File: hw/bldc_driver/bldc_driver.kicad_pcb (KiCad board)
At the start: 4 copper layers, 101 x 48 mm, 150 parts, among them J1 430450412, J2 B4B-EH-A(LF)(SN), J3 B4B-EH-A(LF)(SN), J4 1733583, Q2 IRF540N, Q3 IRF540N, Q4 IRF540N, Q5 IRF540N, Q6 IRF540N, Q7 IRF540N, SW1 BTSA-N-P-1, U1 CH32V30xRxTx, U10 TPS54202DDC, U11 AMC1200BDWV, U12 AMC1200BDWV, U13 AMC1200BDWV, U14 SN65HVD230, U2 STGAP2SCM, U3 STGAP2SCM, U4 STGAP2SCM, U5 STGAP2SCM, U6 STGAP2SCM, U7 STGAP2SCM, U8 TPS54202DDC, U9 AMC1200BDWV, Y1 Crystal_GND24

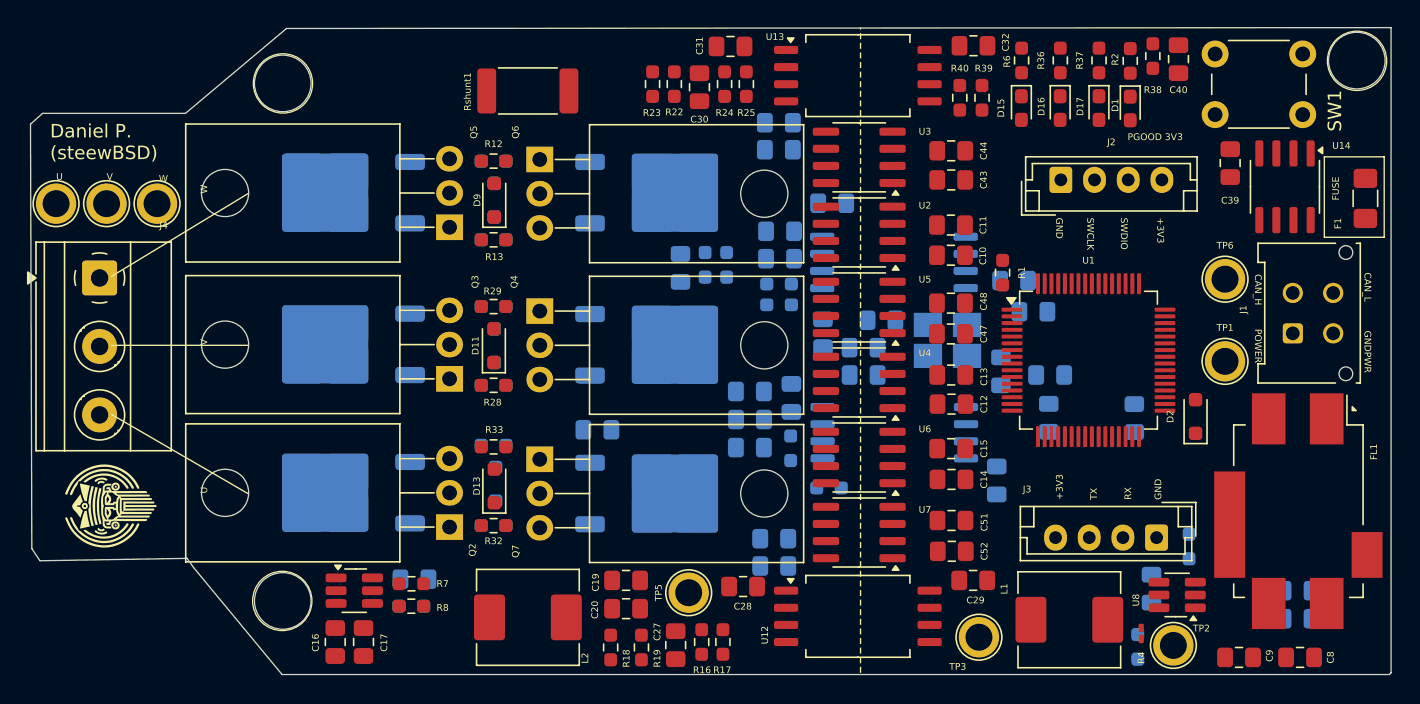
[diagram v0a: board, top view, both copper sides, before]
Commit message: bldc: pre-routing commit
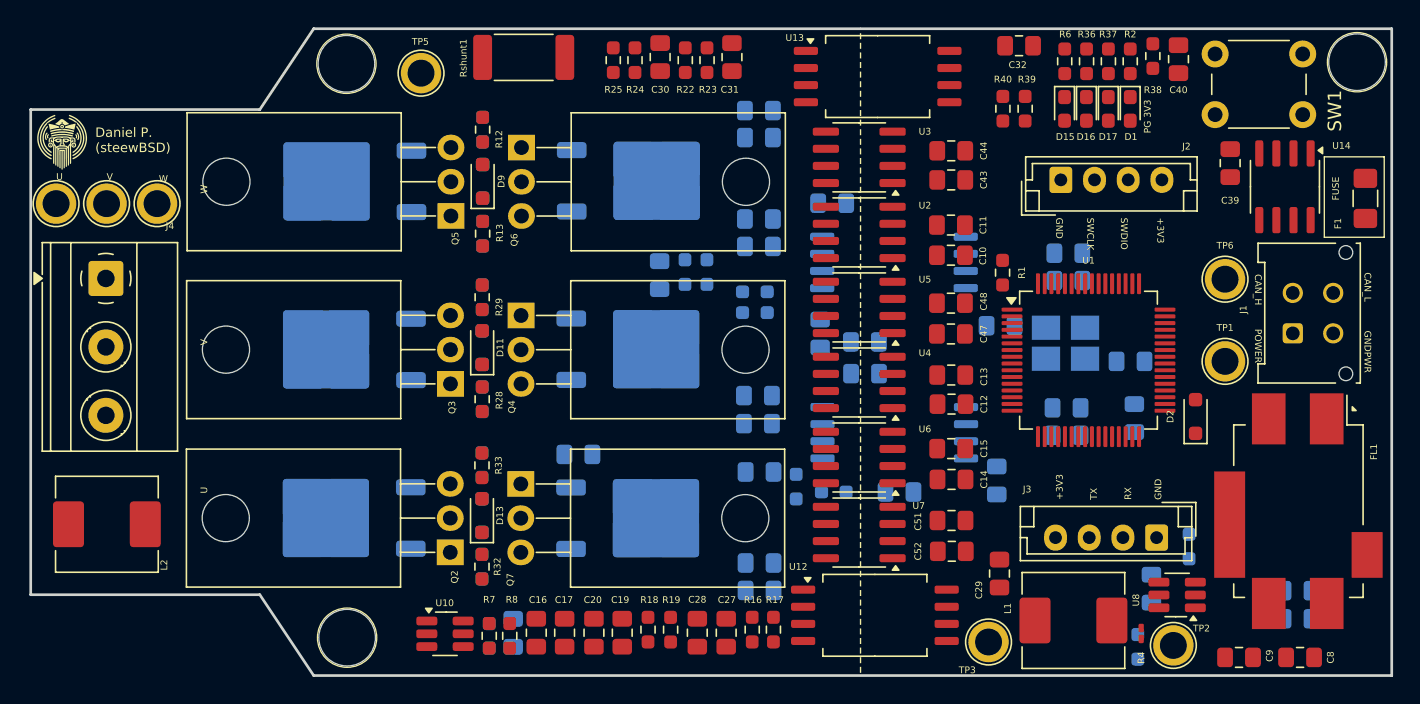
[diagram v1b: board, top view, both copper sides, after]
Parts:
- moved TP5 43.4 mm to (100.5, 70.8)
- moved L2 32.0 mm to (77.2, 104.3)
- moved C16 14.9 mm to (109.0, 112.3)
- moved C17 14.9 mm to (111.1, 112.3)
- moved R25 10.0 mm to (114.7, 69.9), turned to -90 degrees
- moved C42 9.65 mm to (153.1, 92.2), turned to 0 degrees
- moved C21 9.08 mm to (136.0, 101.9)
- moved C41 8.85 mm to (143.5, 89.6)
- moved Y1 8.76 mm to (148.3, 90.9)
- moved C18 8.34 mm to (107.3, 112.3), turned to 90 degrees
- moved R8 7.63 mm to (107.1, 112.6), turned to -90 degrees
- moved U10 7.46 mm to (102.3, 112.4)
- moved R7 6.94 mm to (105.5, 112.6), turned to -90 degrees
- moved R24 6.88 mm to (116.4, 69.9), turned to -90 degrees
- moved R9 6.18 mm to (105.5, 112.6), turned to 90 degrees
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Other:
- outline, holes or cut-outs redrawn
- board text added: "PG 3V3"
- board text removed: "PGOOD 3V3"
